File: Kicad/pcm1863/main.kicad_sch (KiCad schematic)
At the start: 14 parts, among them K101 VCC, U101 AP7375-33, U103 AP7375-33

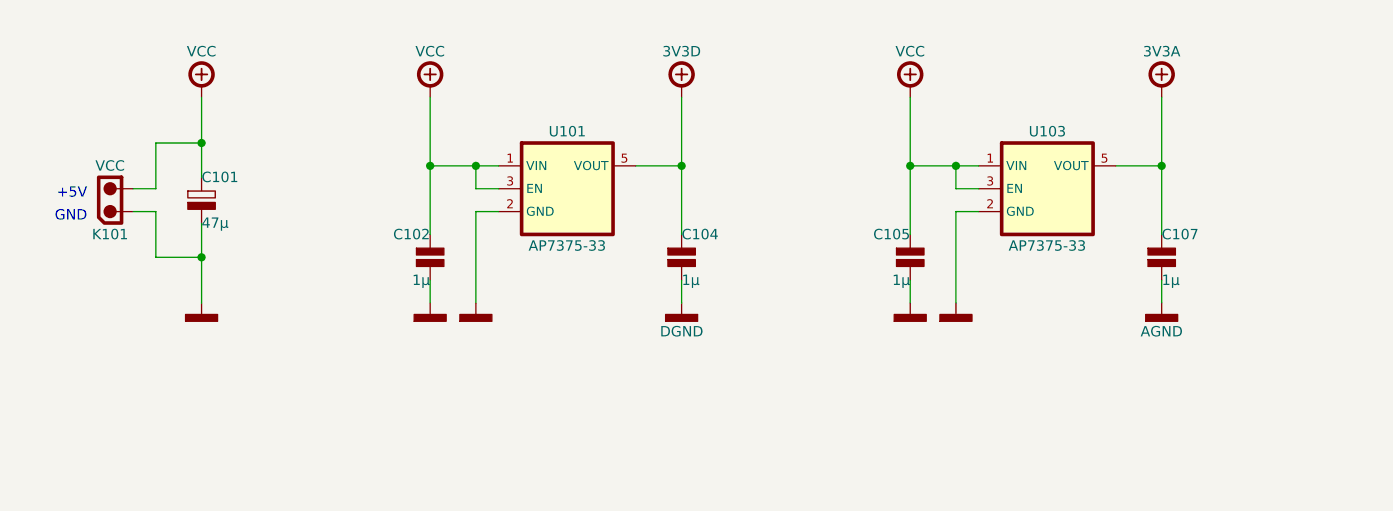
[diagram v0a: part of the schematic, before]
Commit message: Up
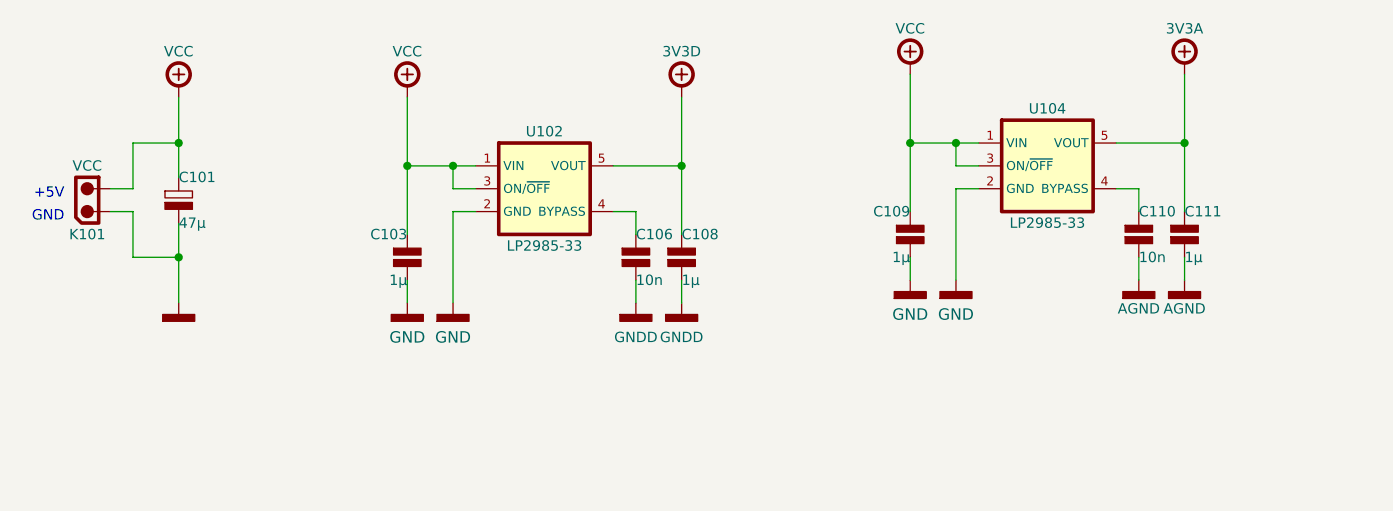
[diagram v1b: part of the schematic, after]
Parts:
- removed C102, C104, C105, C107: 1µ, tronixio:CAPACITOR-SMD-1206, symbol tronixio:CAPACITOR-1206-1U-10P-X7R
- removed U101, U103: AP7375-33, tronixio:SOT25, symbol tronixio:DIODES-AP7375-33-SOT25
- added C103, C108, C109, C111: 1µ, tronixio:CAPACITOR-SMD-1206, symbol tronixio:CAPACITOR-1206-1U-10P-X7R
- added C106, C110: 10n, tronixio:CAPACITOR-SMD-1206, symbol tronixio:CAPACITOR-1206-10N-10P-COG
- added U102, U104: LP2985-33, tronixio:SOT-23-5, symbol tronixio:TI-LP2985-33-SOT23
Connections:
- net +3V3A: now also C111.1, U104.5 (VOUT)
- net +3V3D: now also C108.1, U102.5 (VOUT)
- net AGND: now also C103.2, C109.2, C110.2, C111.2, U102.2 (GND), U104.2 (GND)
- net VCC: now also C103.1, C109.1, U102.1 (VIN), U102.3 (ON/~{OFF}), U104.1 (VIN), U104.3 (ON/~{OFF})
- new net: C106.1, U102.4 (BYPASS)
- new net: C110.1, U104.4 (BYPASS)
- new net GNDD: C106.2, C108.2
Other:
- moved on the sheet: C101, K101
